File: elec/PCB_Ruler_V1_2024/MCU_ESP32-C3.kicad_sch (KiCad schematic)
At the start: 3 parts, among them U2 ESP32-C3-WROOM-02-H4

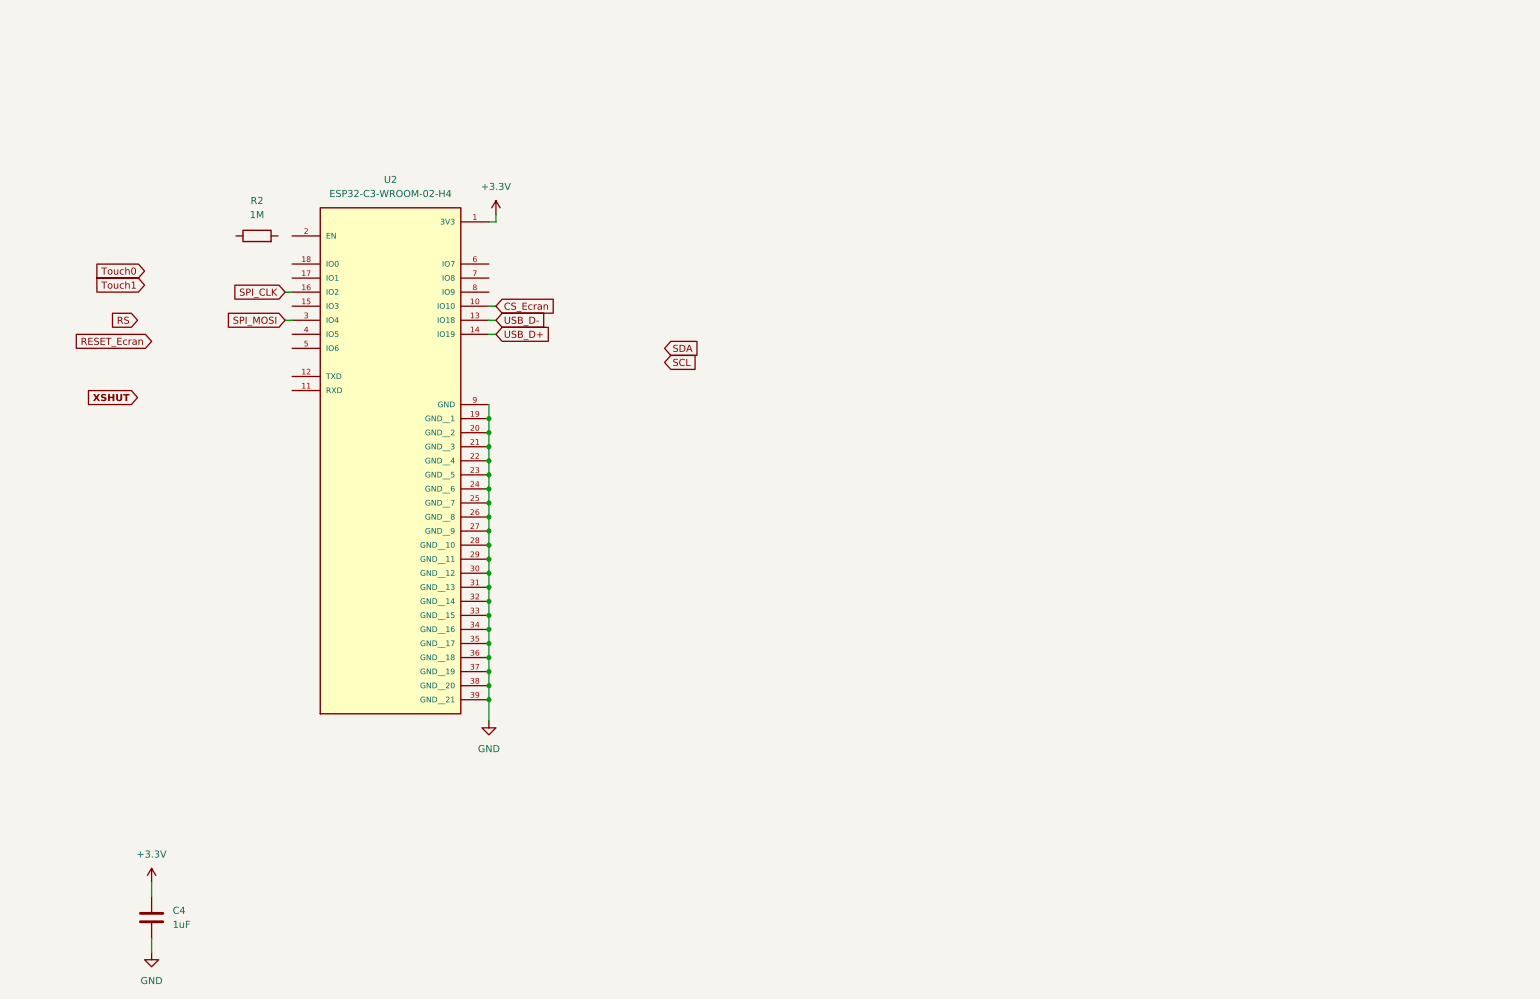
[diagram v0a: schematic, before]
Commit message: Almost finished schematic...
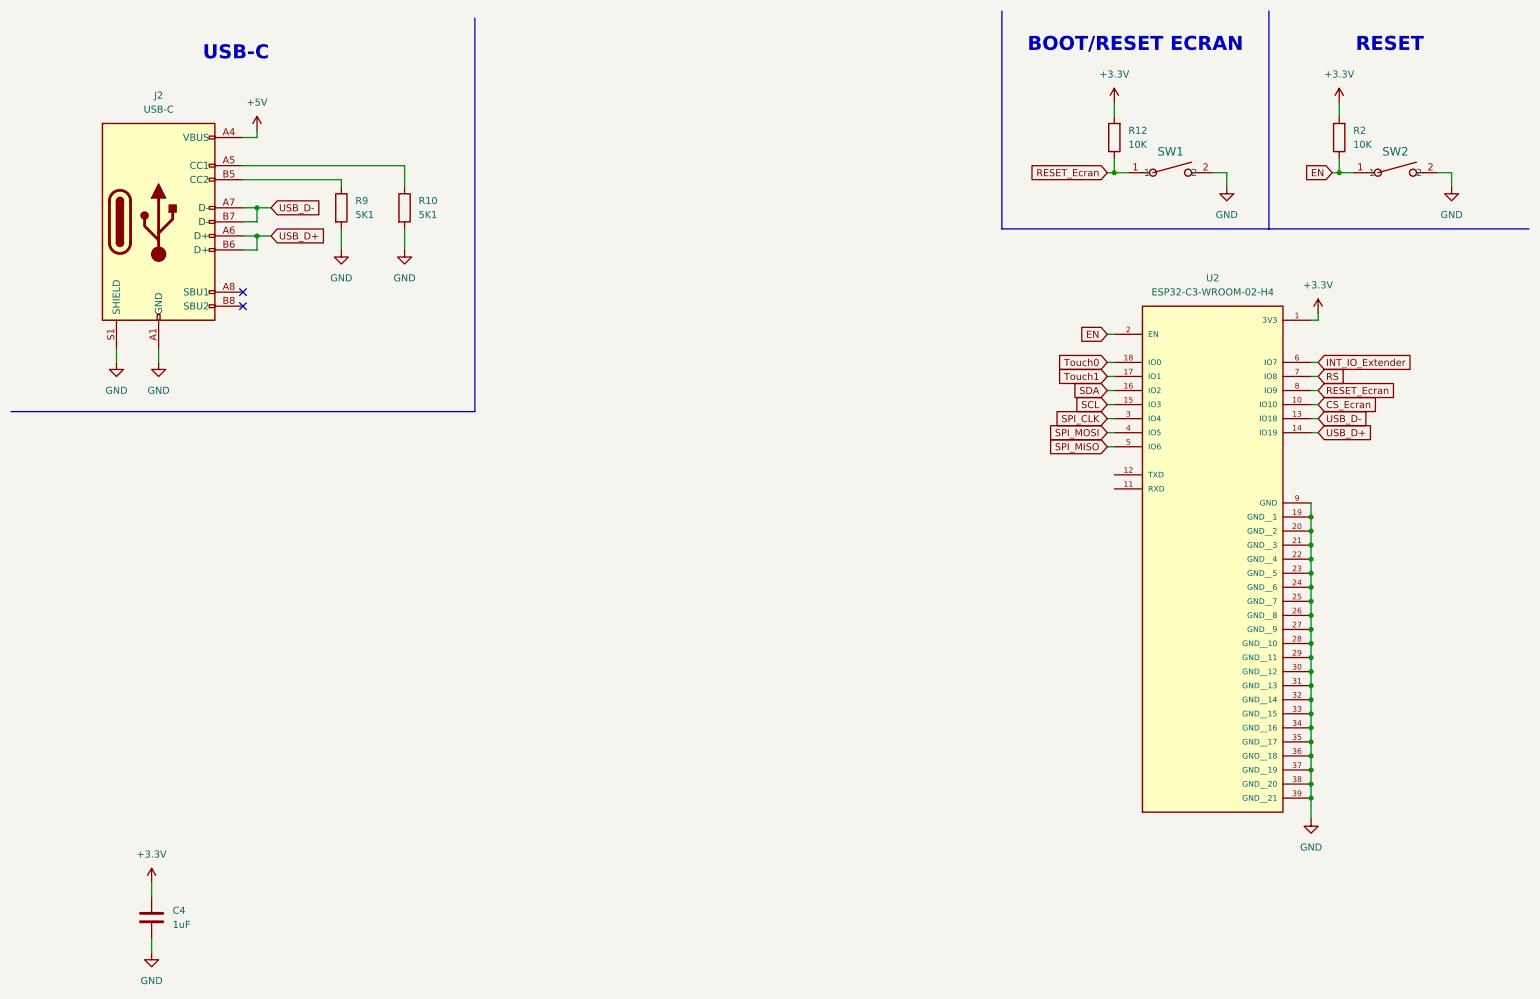
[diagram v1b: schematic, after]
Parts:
- added J2: USB-C, Connector_USB:USB_C_Receptacle_G-Switch_GT-USB-7010ASV, symbol Connector:USB_C_Receptacle_USB2.0_16P
- added R10, R9: 5K1, symbol Device:R
- added R12: 10K, symbol Device:R
- added SW1, SW2: CS1213AGF260, CS1213AGF260:SW_CS1213AGF260_CRS, symbol CS1213AGF260:CS1213AGF260
- R2: value 1M -> 10K
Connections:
- net +3.3V: now also R2.2, R12.2
- net GND: now also J2.A1 (GND), J2.A12 (GND), J2.B1 (GND), J2.B12 (GND), J2.S1 (SHIELD), R10.2, R9.2, SW1.2, SW2.2
- net RESET_Ecran: now also U2.8 (IO9), R12.1, SW1.1
- net RS: now also U2.7 (IO8)
- net SCL: now also U2.15 (IO3)
- net SDA: now also U2.16 (IO2)
- net SPI_CLK: now also U2.3 (IO4); no longer U2.16 (IO2)
- net SPI_MOSI: now also U2.4 (IO5); no longer U2.3 (IO4)
- net Touch0: now also U2.18 (IO0)
- net Touch1: now also U2.17 (IO1)
- net USB_D+: now also J2.A6 (D+), J2.B6 (D+)
- net USB_D-: now also J2.A7 (D-), J2.B7 (D-)
- net EN: now reaches R2.1
- net EN: now also U2.2 (EN), SW2.1
- net SPI_MISO: now reaches U2.5 (IO6)
- net INT_IO_Extender: now reaches U2.6 (IO7)
- new net: J2.B5 (CC2), R9.1
- new net: J2.A5 (CC1), R10.1
- new net +5V: J2.A4 (VBUS), J2.A9 (VBUS), J2.B4 (VBUS), J2.B9 (VBUS)
- no-connect marks 0 -> 2
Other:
- note added: "BOOT/RESET ECRAN"
- note added: "RESET"
- note added: "USB-C"
- moved on the sheet: U2

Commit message: protection and Buttons
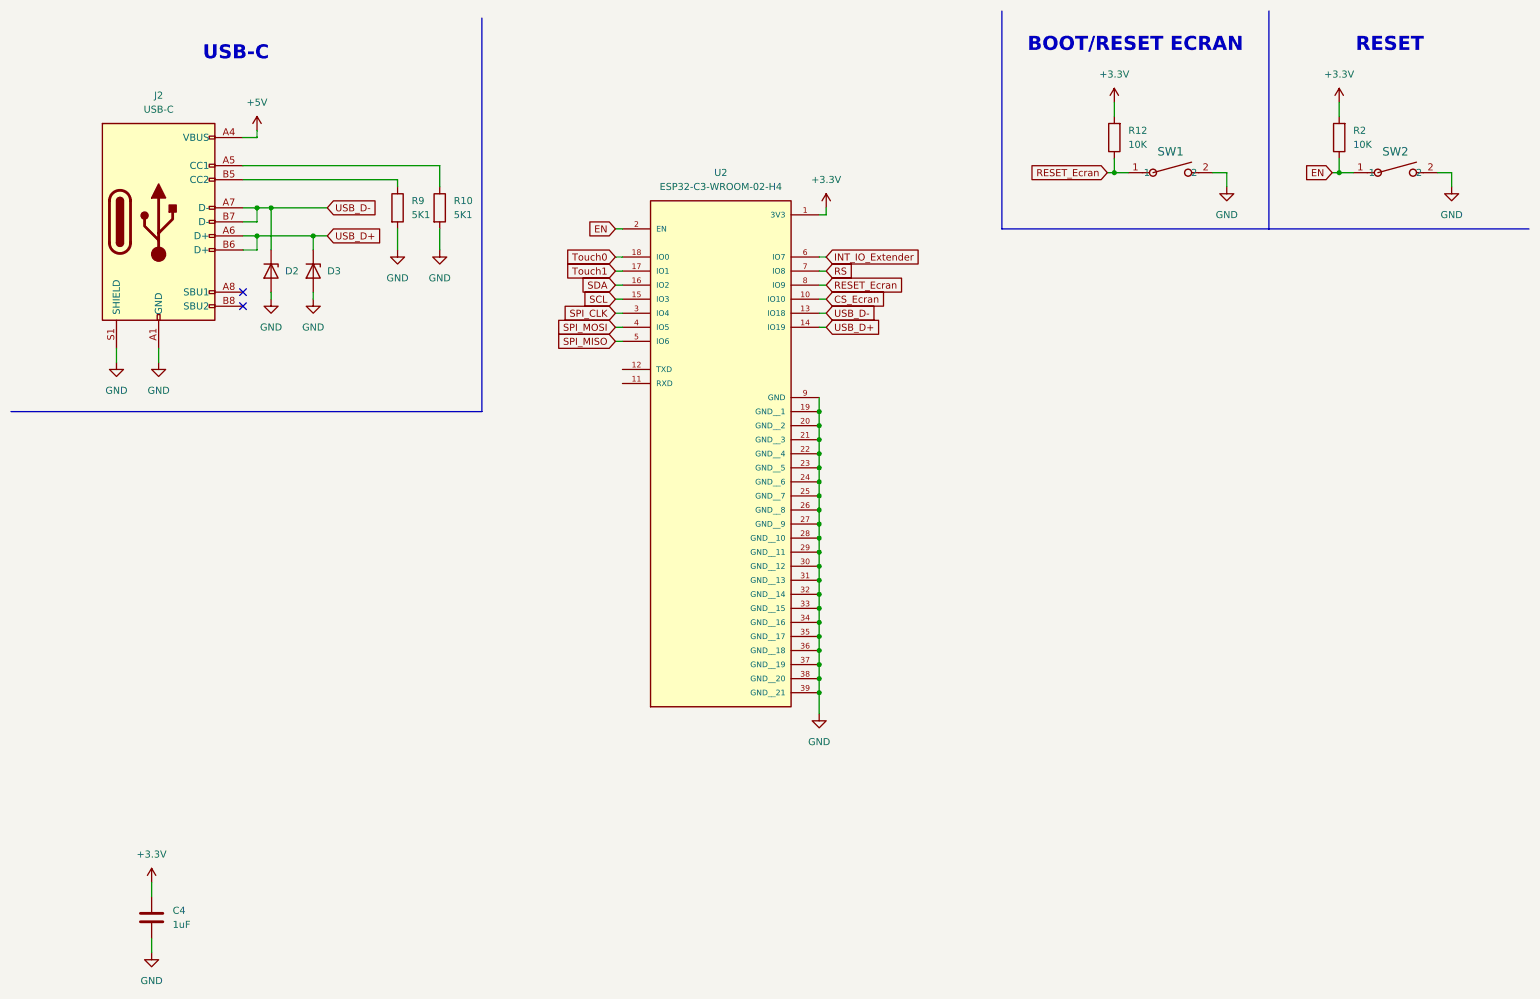
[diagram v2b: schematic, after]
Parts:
- added D2, D3: D_Zener, Diode_SMD:D_SOD-923, symbol Device:D_Zener
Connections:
- net GND: now also D2.2 (A), D3.2 (A)
- net USB_D+: now also D3.1 (K)
- net USB_D-: now also D2.1 (K)
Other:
- moved on the sheet: R10, R9, U2

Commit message: started pcb
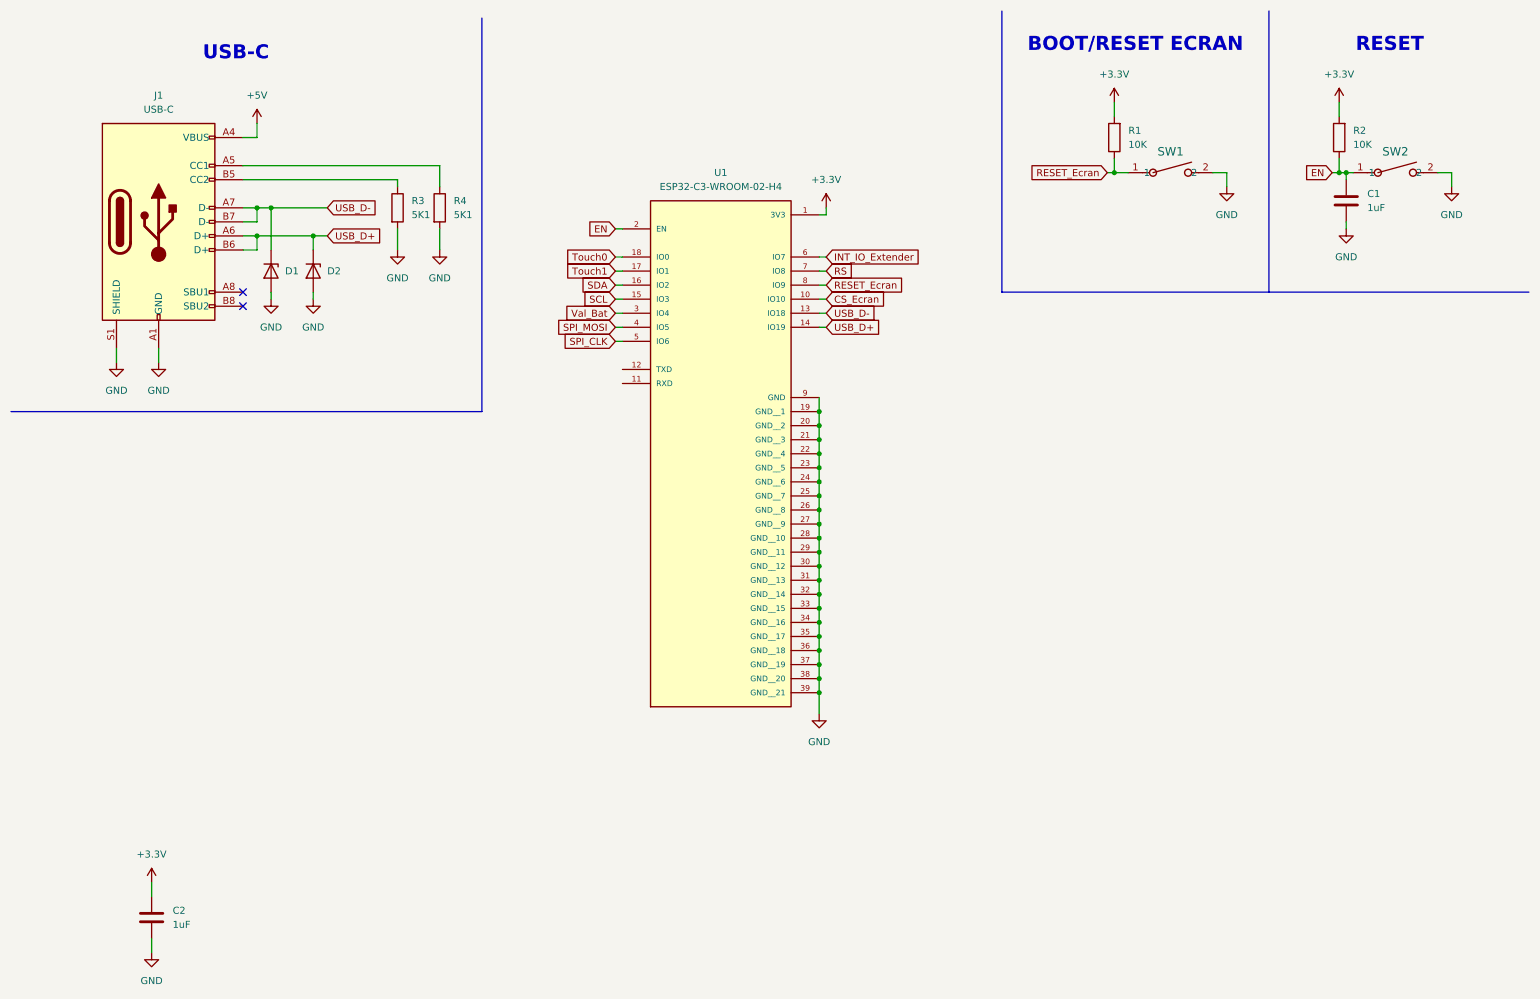
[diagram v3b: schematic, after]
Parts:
- added C1: 1uF, Capacitor_SMD:C_0603_1608Metric_Pad1.08x0.95mm_HandSolder, symbol Device:C
- C2: renamed from C4; footprint (none) -> Capacitor_SMD:C_0603_1608Metric_Pad1.08x0.95mm_HandSolder
- R1: renamed from R12; footprint (none) -> Resistor_SMD:R_0603_1608Metric_Pad0.98x0.95mm_HandSolder
- R2: footprint (none) -> Resistor_SMD:R_0603_1608Metric_Pad0.98x0.95mm_HandSolder
- R3: renamed from R9; footprint (none) -> Resistor_SMD:R_0603_1608Metric_Pad0.98x0.95mm_HandSolder
- R4: renamed from R10; footprint (none) -> Resistor_SMD:R_0603_1608Metric_Pad0.98x0.95mm_HandSolder
- renumbered D2 to D1, D3 to D2, J2 to J1, U2 to U1
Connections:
- net SPI_MISO is gone; now on net SPI_CLK: U1.5 (IO6)
- net EN: now also C1.1
- net GND: now also C1.2
- net SPI_CLK: no longer U1.3 (IO4)
- new net Val_Bat: U1.3 (IO4)
